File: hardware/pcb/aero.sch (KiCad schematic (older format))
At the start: 2 parts

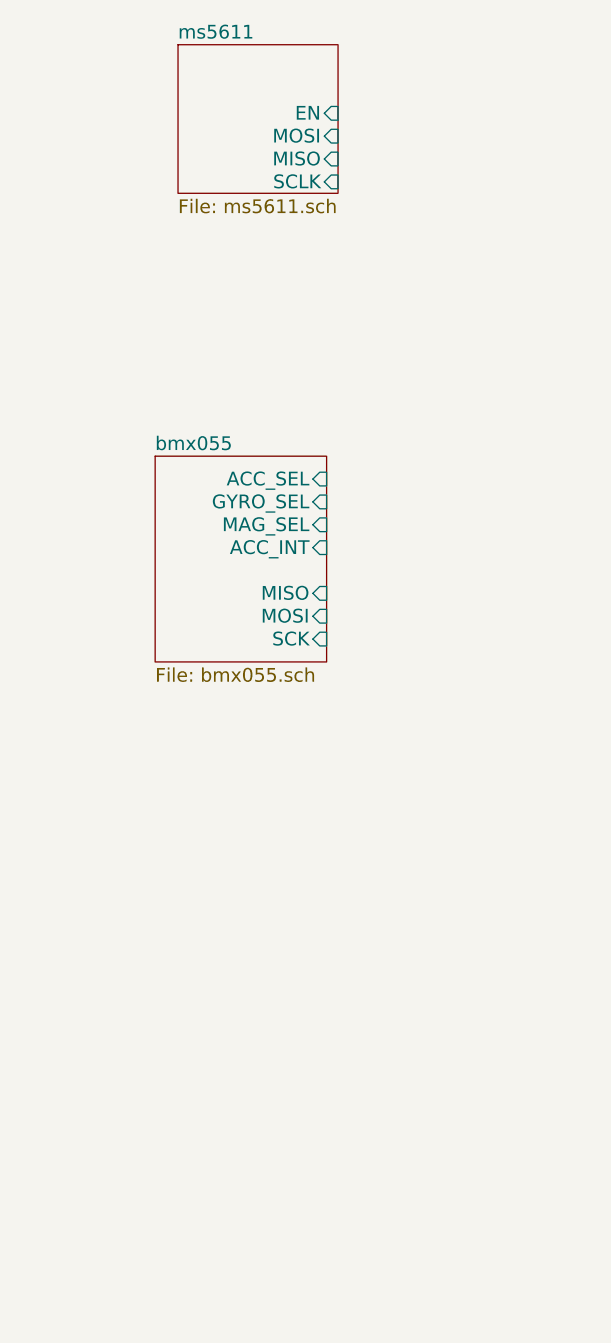
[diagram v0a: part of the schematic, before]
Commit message: more progress on hw
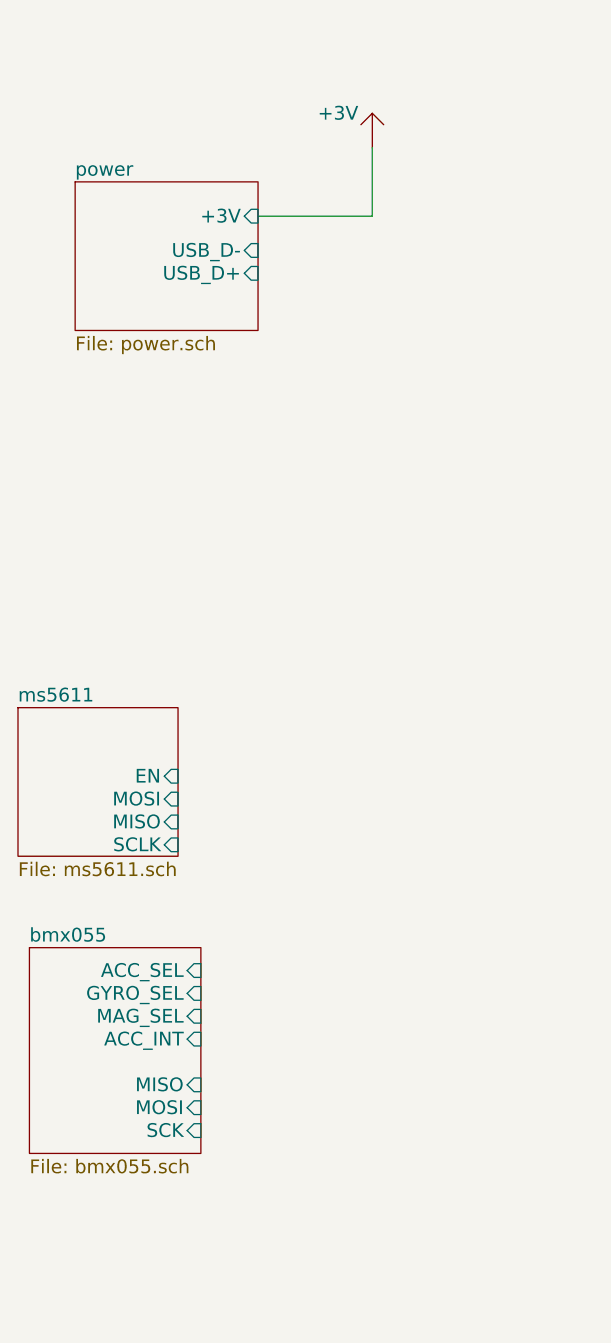
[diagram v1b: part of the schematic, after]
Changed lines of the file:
@@
 $Descr A4 11693 8268
 encoding utf-8
-Sheet 1 5
+Sheet 1 6
 Title ""
 Date ""
@@
 $EndSheet
 $Sheet
-S 1950 850  700  650
+S 1250 3750 700  650
 U 551EEA41
 F0 "ms5611" 60
 F1 "ms5611.sch" 60
-F2 "EN" I R 2650 1150 60
-F3 "SCLK" I R 2650 1450 60
-F4 "MOSI" I R 2650 1250 60
-F5 "MISO" I R 2650 1350 60
-$EndSheet
-$Sheet
-S 1850 2650 750  900
+F2 "EN" I R 1950 4050 60
+F3 "SCLK" I R 1950 4350 60
+F4 "MOSI" I R 1950 4150 60
+F5 "MISO" I R 1950 4250 60
+$EndSheet
+$Sheet
+S 1300 4800 750  900
 U 5527E8E0
 F0 "bmx055" 60
 F1 "bmx055.sch" 60
-F2 "ACC_SEL" I R 2600 2750 60
-F3 "GYRO_SEL" I R 2600 2850 60
-F4 "MAG_SEL" I R 2600 2950 60
-F5 "ACC_INT" I R 2600 3050 60
-F6 "MISO" I R 2600 3250 60
-F7 "MOSI" I R 2600 3350 60
-F8 "SCK" I R 2600 3450 60
+F2 "ACC_SEL" I R 2050 4900 60
+F3 "GYRO_SEL" I R 2050 5000 60
+F4 "MAG_SEL" I R 2050 5100 60
+F5 "ACC_INT" I R 2050 5200 60
+F6 "MISO" I R 2050 5400 60
+F7 "MOSI" I R 2050 5500 60
+F8 "SCK" I R 2050 5600 60
 $EndSheet
 $Comp
@@
 	9100 2600 9100 3900
 Connection ~ 9100 3900
+$Sheet
+S 1500 1450 800  650
+U 552EDA4D
+F0 "power" 60
+F1 "power.sch" 60
+F2 "+3V" I R 2300 1600 60
+F3 "USB_D-" I R 2300 1750 60
+F4 "USB_D+" I R 2300 1850 60
+$EndSheet
+$Comp
+L +3V #PWR?
+U 1 1 552F0919
+P 2800 1300
+F 0 "#PWR?" H 2800 1200 60  0001 C CNN
+F 1 "+3V" H 2650 1450 60  0000 C CNN
+F 2 "" H 2800 1300 60  0000 C CNN
+F 3 "" H 2800 1300 60  0000 C CNN
+	1    2800 1300
+	1    0    0    -1
+$EndComp
+Wire Wire Line
+	2800 1300 2800 1600
+Wire Wire Line
+	2800 1600 2300 1600
 $EndSCHEMATC
